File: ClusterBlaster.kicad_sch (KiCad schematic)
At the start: 14 parts, among them J1 Conn_01x04, J2 Conn_01x03, U1 LM339, U2 L7805, U3 ARDUINO_PRO_MINI

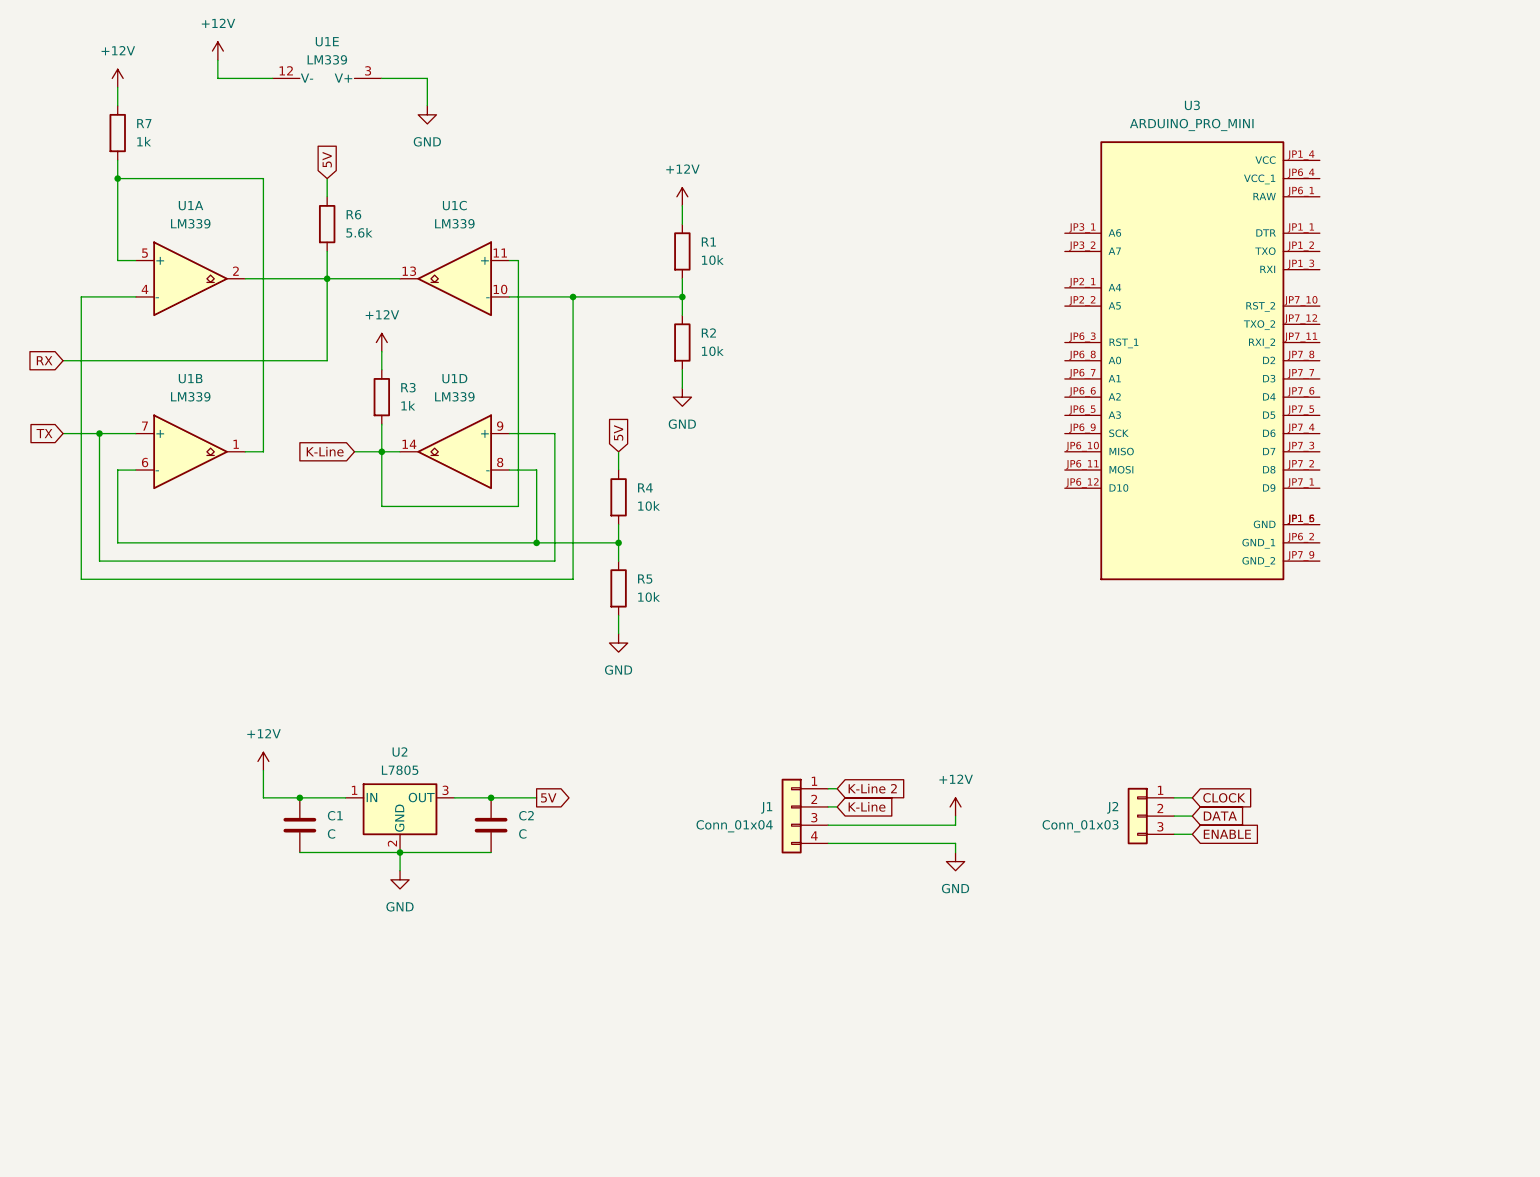
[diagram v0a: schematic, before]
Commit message: Added all the components
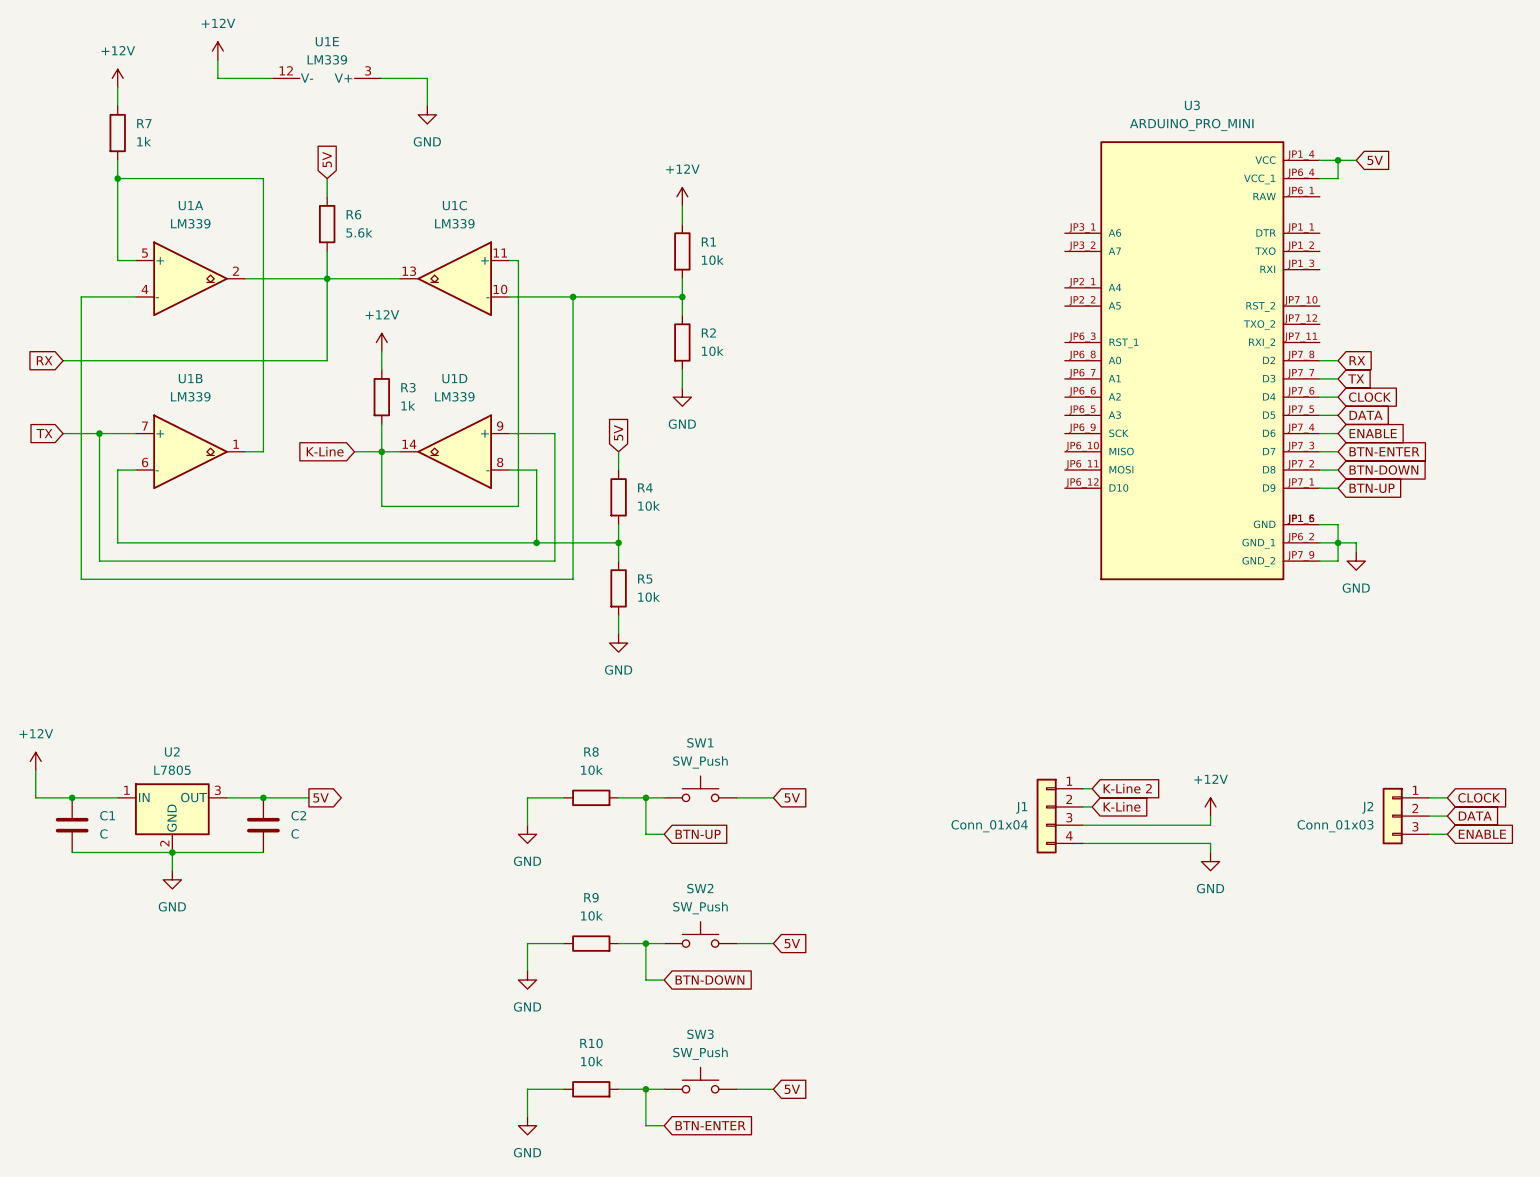
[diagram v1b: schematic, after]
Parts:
- added R10, R8, R9: 10k, Resistor_SMD:R_0805_2012Metric, symbol Device:R
- added SW1, SW2, SW3: SW_Push, Button_Switch_THT:SW_PUSH_6mm, symbol Switch:SW_Push
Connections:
- net 5V: now also U3.JP1_4 (VCC), U3.JP6_4 (VCC_1), SW1.2, SW2.2, SW3.2
- net CLOCK: now also U3.JP7_6 (D4)
- net DATA: now also U3.JP7_5 (D5)
- net ENABLE: now also U3.JP7_4 (D6)
- net GND: now also U3.JP1_5 (GND), U3.JP1_6 (GND), U3.JP6_2 (GND_1), U3.JP7_9 (GND_2), R10.1, R8.1, R9.1
- net RX: now also U3.JP7_8 (D2)
- net TX: now also U3.JP7_7 (D3)
- net BTN-UP: now reaches U3.JP7_1 (D9)
- net BTN-UP: now also R8.2, SW1.1
- net BTN-DOWN: now reaches U3.JP7_2 (D8)
- net BTN-DOWN: now also R9.2, SW2.1
- net BTN-ENTER: now reaches U3.JP7_3 (D7)
- net BTN-ENTER: now also R10.2, SW3.1
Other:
- moved on the sheet: C1, C2, J1, J2, U2
